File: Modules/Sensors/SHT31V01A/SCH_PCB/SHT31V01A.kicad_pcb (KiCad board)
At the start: 2 copper layers, 40.1 x 9.7 mm, 18 parts, among them J1 CONN1_1, J10 JUMP_2x1, J11 JUMP_2x1, J12 JUMP_2x1, J13 JUMP_2x1, J2 CONN1_1, J9 JUMP_2x1, M1 HOLE, M2 HOLE, U1 SHT31

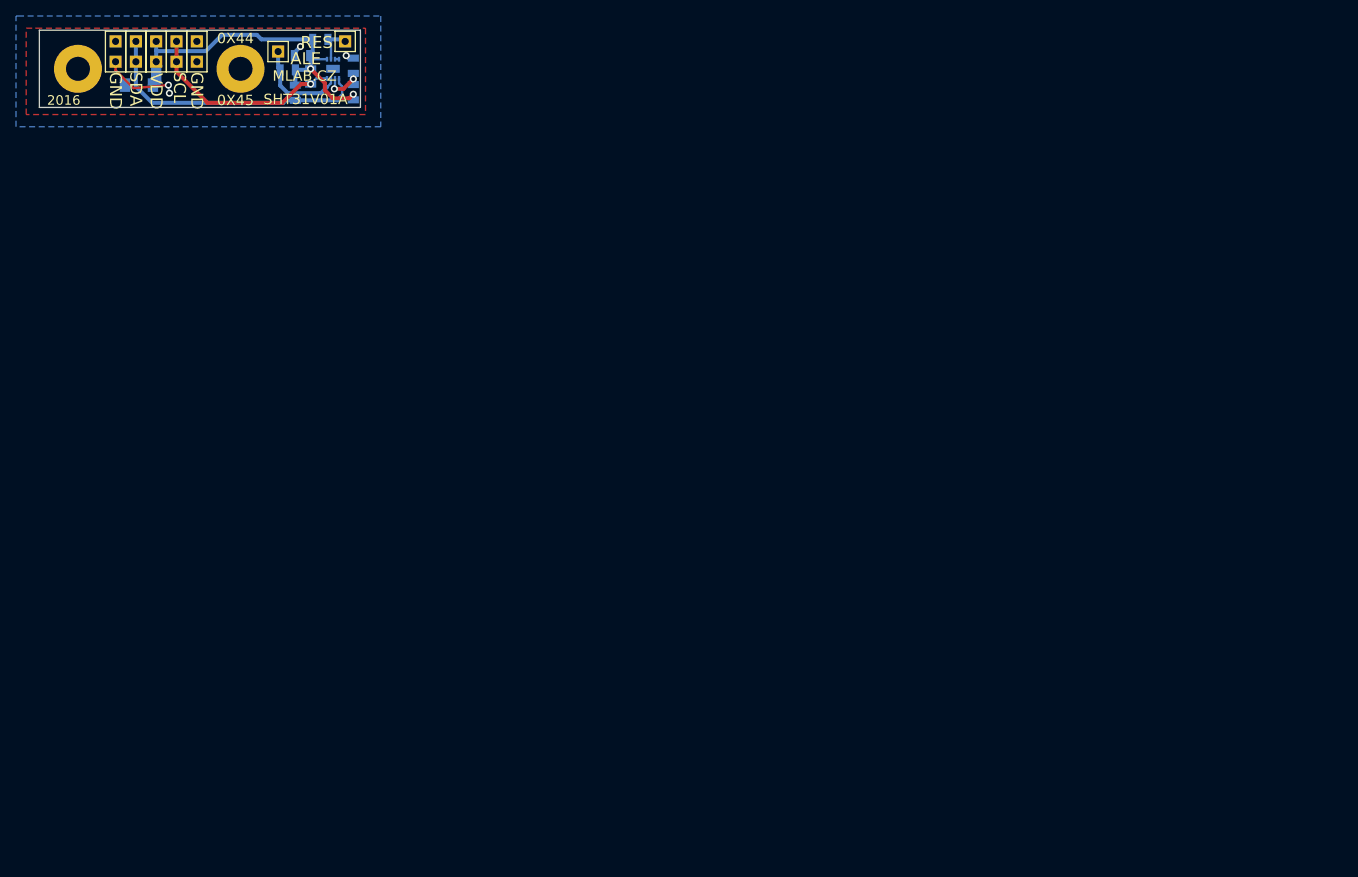
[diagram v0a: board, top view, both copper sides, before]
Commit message: Nahrani dokumentace
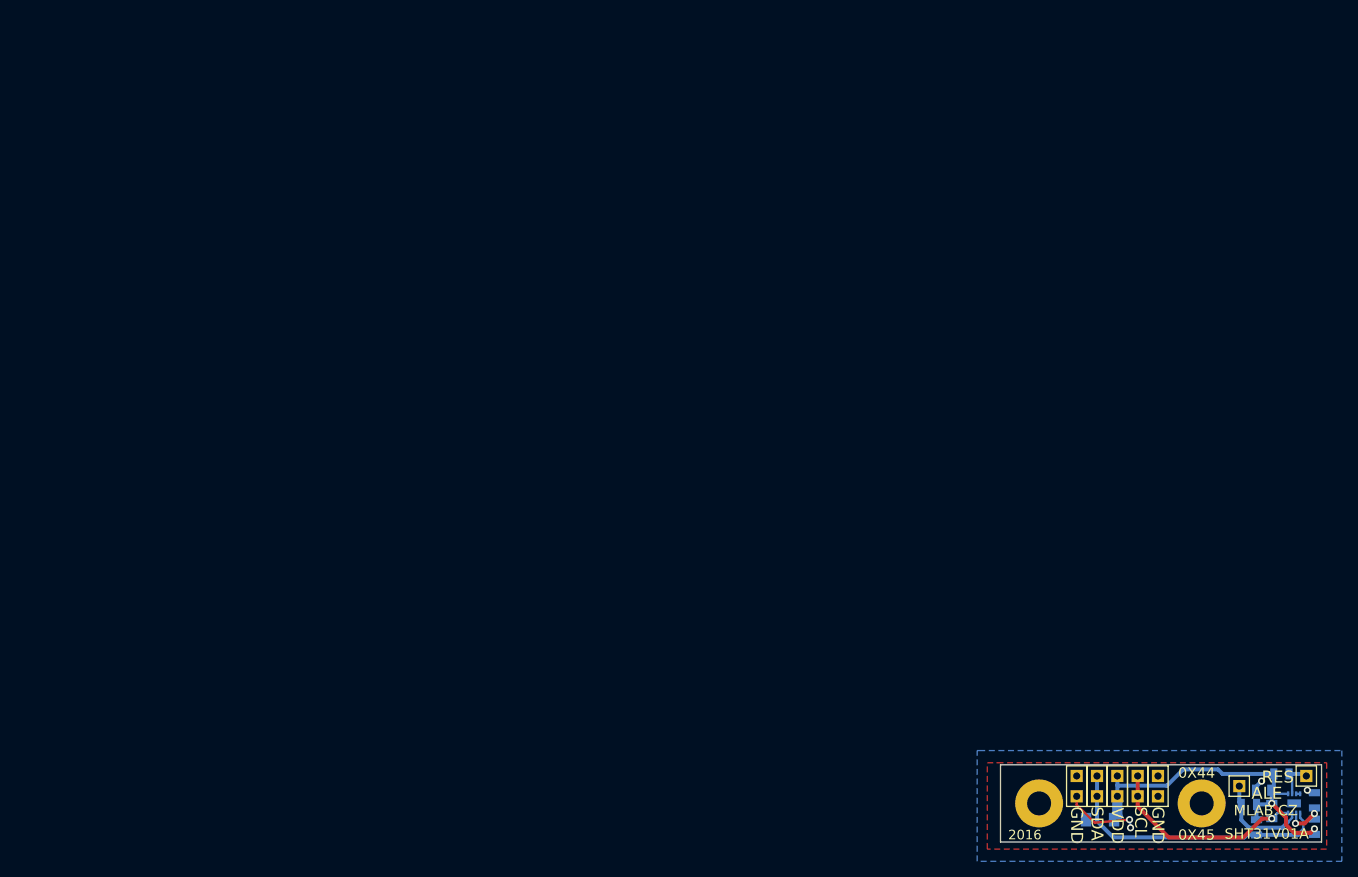
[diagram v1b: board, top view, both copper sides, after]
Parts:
- D1: value BZV55C-3,6V -> BZV55C-5,6V
- moved J11 151.2 mm to (137.5, 84.6)
- moved J12 151.2 mm to (129.9, 84.6)
- moved J13 151.2 mm to (140.1, 84.6)
- moved J2 151.2 mm to (158.6, 83.3)
- moved M1 151.2 mm to (145.5, 86.7)
- moved M2 151.2 mm to (125.2, 86.7)
- moved R1 151.2 mm to (151.4, 86.9)
- moved R2 151.2 mm to (155.5, 83.1)
- moved R3 151.2 mm to (159.6, 89.7)
- moved R5 151.2 mm to (152.4, 89.7)
- moved U1 151.2 mm to (157.1, 86.7)
- moved C1 151.2 mm to (153.2, 85.1)
- moved D1 151.2 mm to (132.8, 88.8)
- moved J1 151.2 mm to (150.2, 84.6)
- moved J10 151.2 mm to (132.5, 84.6)
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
